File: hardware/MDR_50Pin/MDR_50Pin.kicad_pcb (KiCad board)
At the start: 2 copper layers, 59.9 x 82.5 mm, 72 parts, among them J2 TRM_BCKF, Q3 AO3401A, U10 Centronics50PinMale, U3 AP1117-ADJ, U4 LVTH245, U5 LVT125, U6 LVT125, U7 LVT125, U8 74HC14, U9 LVTH245

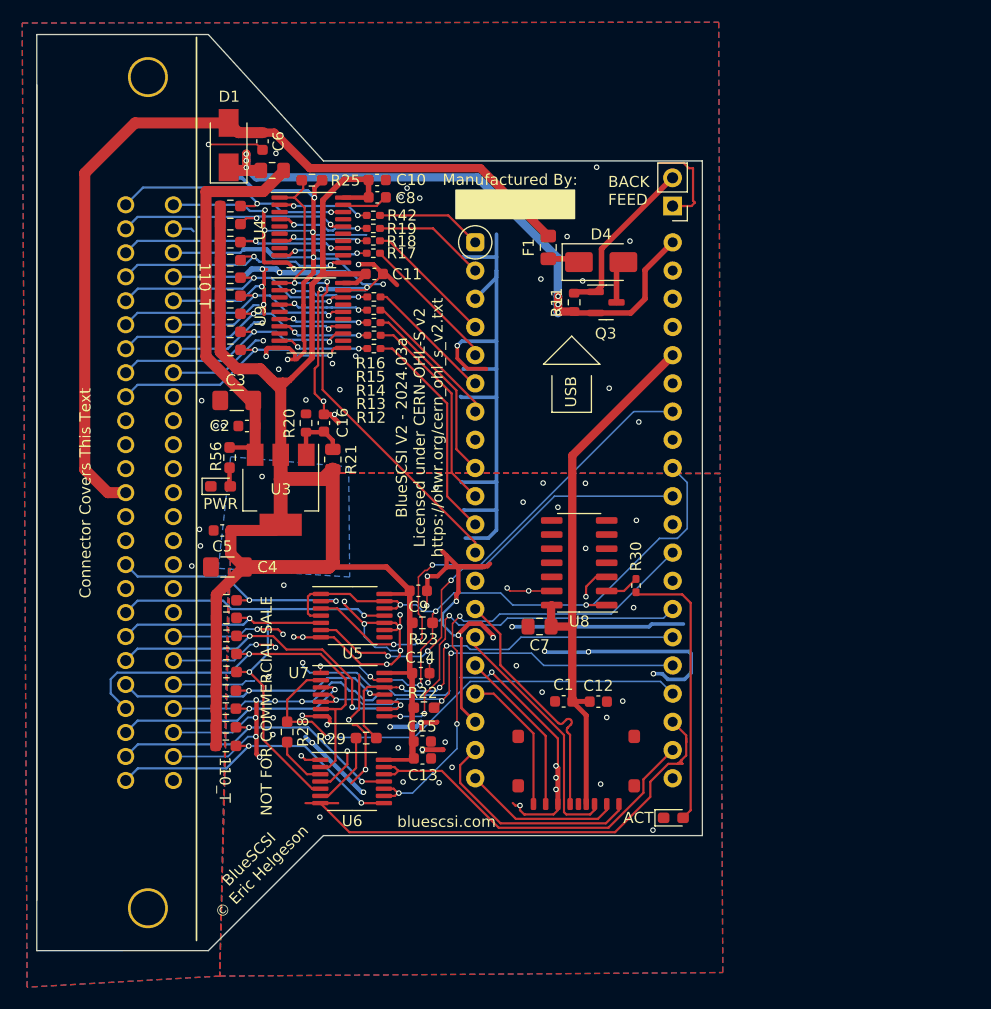
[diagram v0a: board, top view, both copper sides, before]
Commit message: latest design
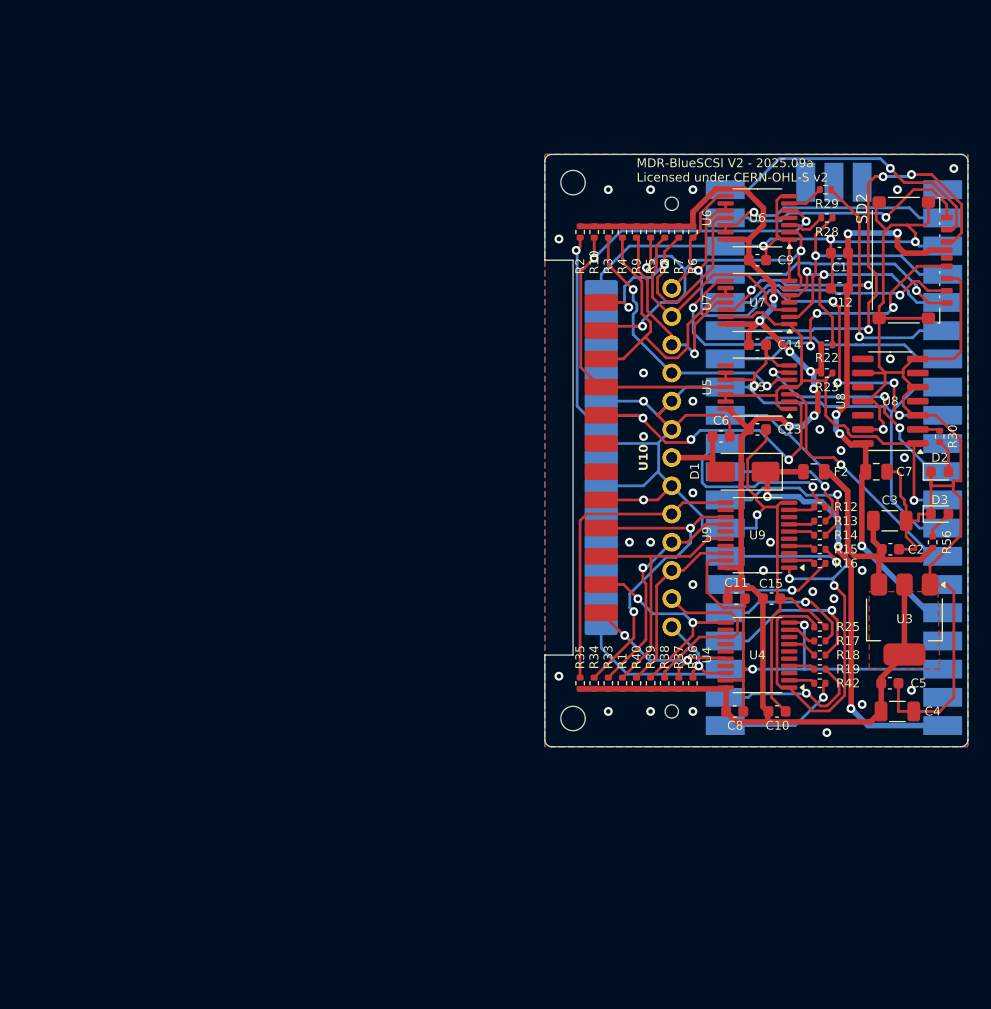
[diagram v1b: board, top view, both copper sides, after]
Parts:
- removed C16: 10uF, Capacitor_SMD:C_0603_1608Metric
- removed D4: D, Diode_SMD:D_SMA
- removed F1: Polyfuse, Fuse:Fuse_0805_2012Metric_Pad1.15x1.40mm_HandSolder
- removed G***: LOGO, LOGO
- removed J2: TRM_BCKF, Connector_PinHeader_2.54mm:PinHeader_1x02_P2.54mm_Vertical
- removed Q3: AO3401A, Package_TO_SOT_SMD:SOT-23
- removed R11: 10k, Resistor_SMD:R_0603_1608Metric
- removed R20: 154, Resistor_SMD:R_0603_1608Metric
- removed R21: 120, Resistor_SMD:R_0805_2012Metric
- added REF**: MountingHole_2.2mm_M2_ISO7380, MountingHole:MountingHole_2.2mm_M2_ISO7380, F.Cu at (137.8, 73.0)
- added REF**: MountingHole_2.2mm_M2_ISO7380, MountingHole:MountingHole_2.2mm_M2_ISO7380, F.Cu at (137.8, 121.3)
- C3, C4: footprint Capacitor_SMD:C_1206_3216Metric_Pad1.42x1.75mm_HandSolder -> Capacitor_SMD:C_1206_3216Metric
- C7: footprint Capacitor_SMD:C_0805_2012Metric_Pad1.18x1.45mm_HandSolder -> Capacitor_SMD:C_0805_2012Metric
- D2, D3: footprint LED_SMD:LED_0603_1608Metric_Pad1.05x0.95mm_HandSolder -> LED_SMD:LED_0603_1608Metric
- F2: footprint Fuse:Fuse_0805_2012Metric_Pad1.15x1.40mm_HandSolder -> Fuse:Fuse_0805_2012Metric
- R1, R10, R2, R22, R23, R25, R28, R29, R3, R33, R34, R35, R36, R37, R38, R39, R4, R40, R5, R56, R6, R7, R8, R9: footprint Resistor_SMD:R_0603_1608Metric_Pad0.98x0.95mm_HandSolder -> Resistor_SMD:R_0402_1005Metric
- R12, R13, R14, R15, R16, R17, R18, R19, R30, R42: footprint Resistor_SMD:R_0402_1005Metric_Pad0.72x0.64mm_HandSolder -> Resistor_SMD:R_0402_1005Metric
- RP1: footprint CustomFootprints:BluePillModule -> Library:RPi_Pico_SMD; moved to B.Cu
- SD2: footprint Library:TF-06_MicroSD -> Library:TF-SMD_TF-06A
- U10: value Centronics50PinMale -> MDR50; footprint Library:Centronics50Male -> Library:MDR50
- U3: value AP1117-ADJ -> AMS1117-2.85
- moved R28 67.1 mm to (160.7, 76.2), turned to 180 degrees
- moved D3 64.8 mm to (170.8, 102.9)
- moved R29 64.4 mm to (160.5, 73.7)
- moved R56 63.8 mm to (170.2, 105.4), turned to 90 degrees
- moved R6 62.5 mm to (148.6, 77.5), turned to 90 degrees
- moved U6 62.5 mm to (154.4, 76.2), turned to 180 degrees
- moved C4 61.7 mm to (167.0, 120.7), turned to 0 degrees
- moved C5 61.7 mm to (166.3, 118.1), turned to 0 degrees
- moved R25 60.9 mm to (160.0, 113.0)
- moved R7 60.4 mm to (147.3, 77.5), turned to 90 degrees
- moved C10 59.9 mm to (156.2, 120.7)
- moved R36 59.9 mm to (148.6, 118.1), turned to -90 degrees
- moved C3 59.8 mm to (166.3, 103.5), turned to 0 degrees
- moved C2 59.0 mm to (166.4, 106.0), turned to 0 degrees
- moved R8 58.4 mm to (146.1, 77.5), turned to 90 degrees
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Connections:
- U3 pad 1: Net-(U3-ADJ) -> GND
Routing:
- net GND: track 540.7 -> 390.4 mm, vias 118 -> 39
- net +5V: track 79.1 -> 7.17 mm
- net oBSY: track 70.5 -> 45.0 mm, vias 6 -> 1
- net ATN: track 22.9 -> 47.8 mm, vias 2 -> 4
- net iATN: track 45.5 -> 21.7 mm, vias 3 -> 1
- net Net-(D2-A): track 25.0 -> 2.99 mm
- net oCD_iSEL: track 43.6 -> 22.2 mm
- net iACK: track 41.3 -> 20.9 mm
- net +5VP: track 58.1 -> 38.3 mm, vias 6 -> 3
- net SD_CMD_MOSI: track 22.6 -> 41.8 mm, vias 0 -> 3
- net IO: track 27.9 -> 10.7 mm, vias 2 -> 0
- net oSEL: track 39.2 -> 23.5 mm, vias 3 -> 2
- net Net-(J2-Pin_2): track 15.1 -> 0.00 mm
- net +2V8: track 152.8 -> 137.7 mm, vias 0 -> 7
- net DB0: track 23.1 -> 8.48 mm, vias 2 -> 1
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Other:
- board size 59.9 x 82.5 mm -> 38.1 x 53.3 mm
- board text added: "Derived from BlueSCSI V2"
- board text added: "MDR-BlueSCSI V2 - 2025.09a Licensed under CERN-OHL-S v2"
- board text removed: "110_T"
- board text removed: "ACT"
- board text removed: "BACK FEED"
- board text removed: "BlueSCSI V2 - 2024.03a Licensed under CERN-OHL-S v2 https://ohwr.org/cern_ohl_s_v2.txt"
- board text removed: "BlueSCSI © Eric Helgeson"
- board text removed: "Connector Covers This Text"
- board text removed: "Manufactured By:"
- board text removed: "NOT FOR COMMERCIAL SALE"
- board text removed: "PCB © Tech by Androda, LLC"
- board text removed: "PWR"
- board text removed: "bluescsi.com"
